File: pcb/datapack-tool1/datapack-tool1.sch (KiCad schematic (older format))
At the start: 4 parts

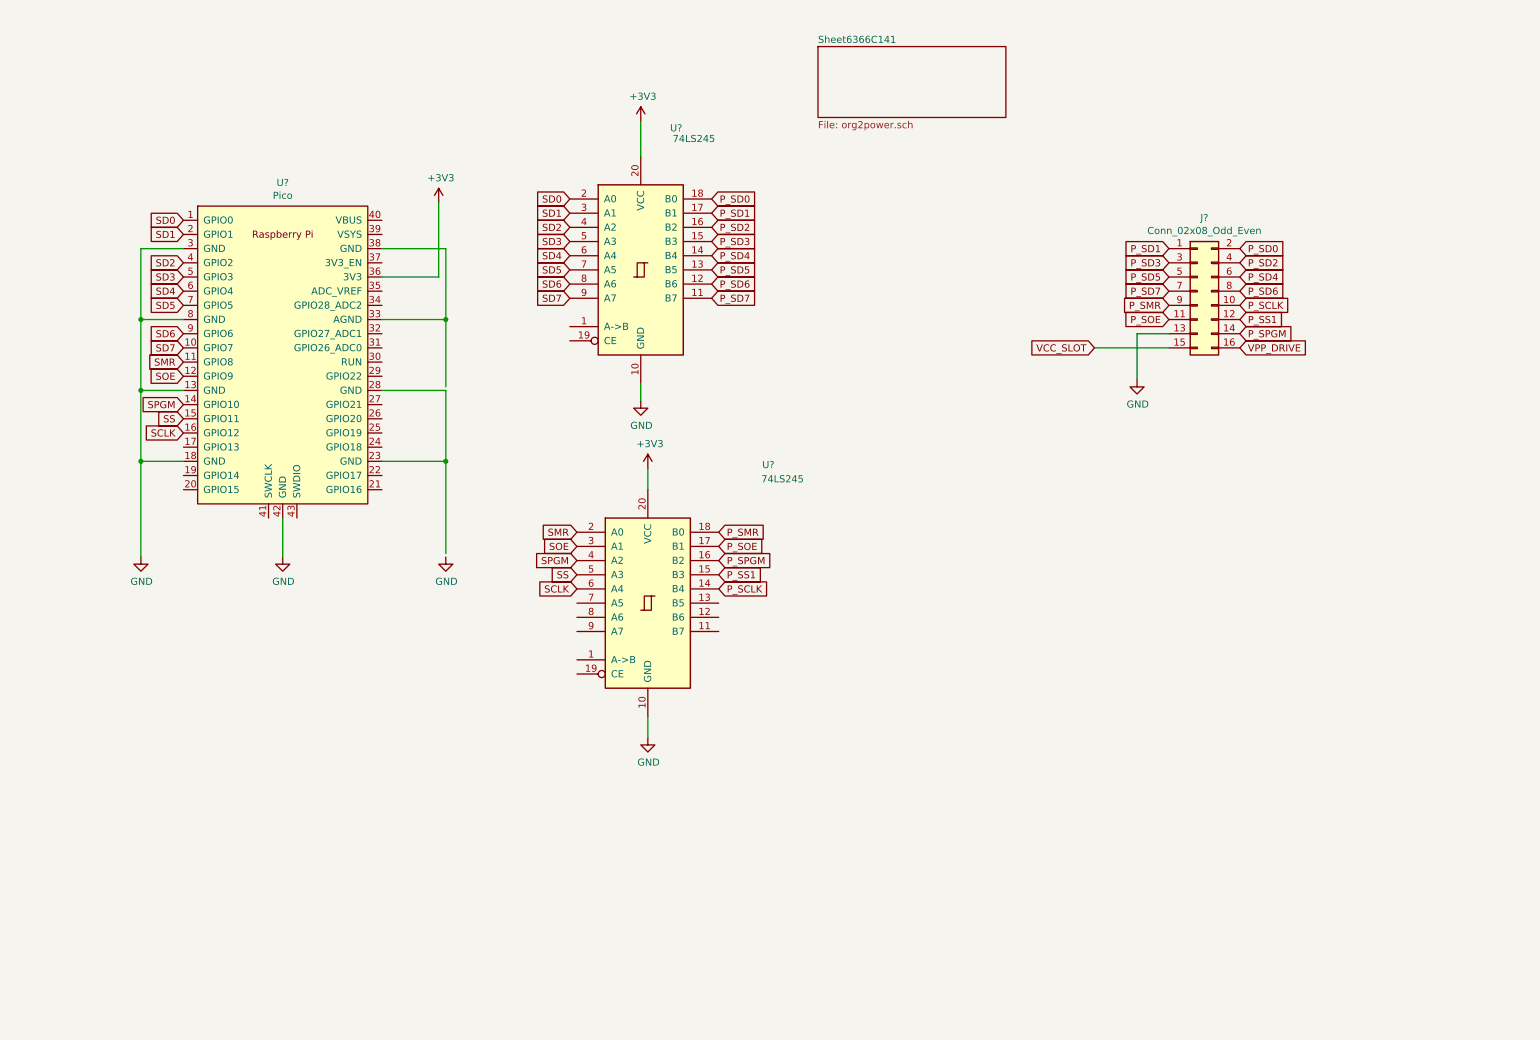
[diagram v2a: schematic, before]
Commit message: Updates
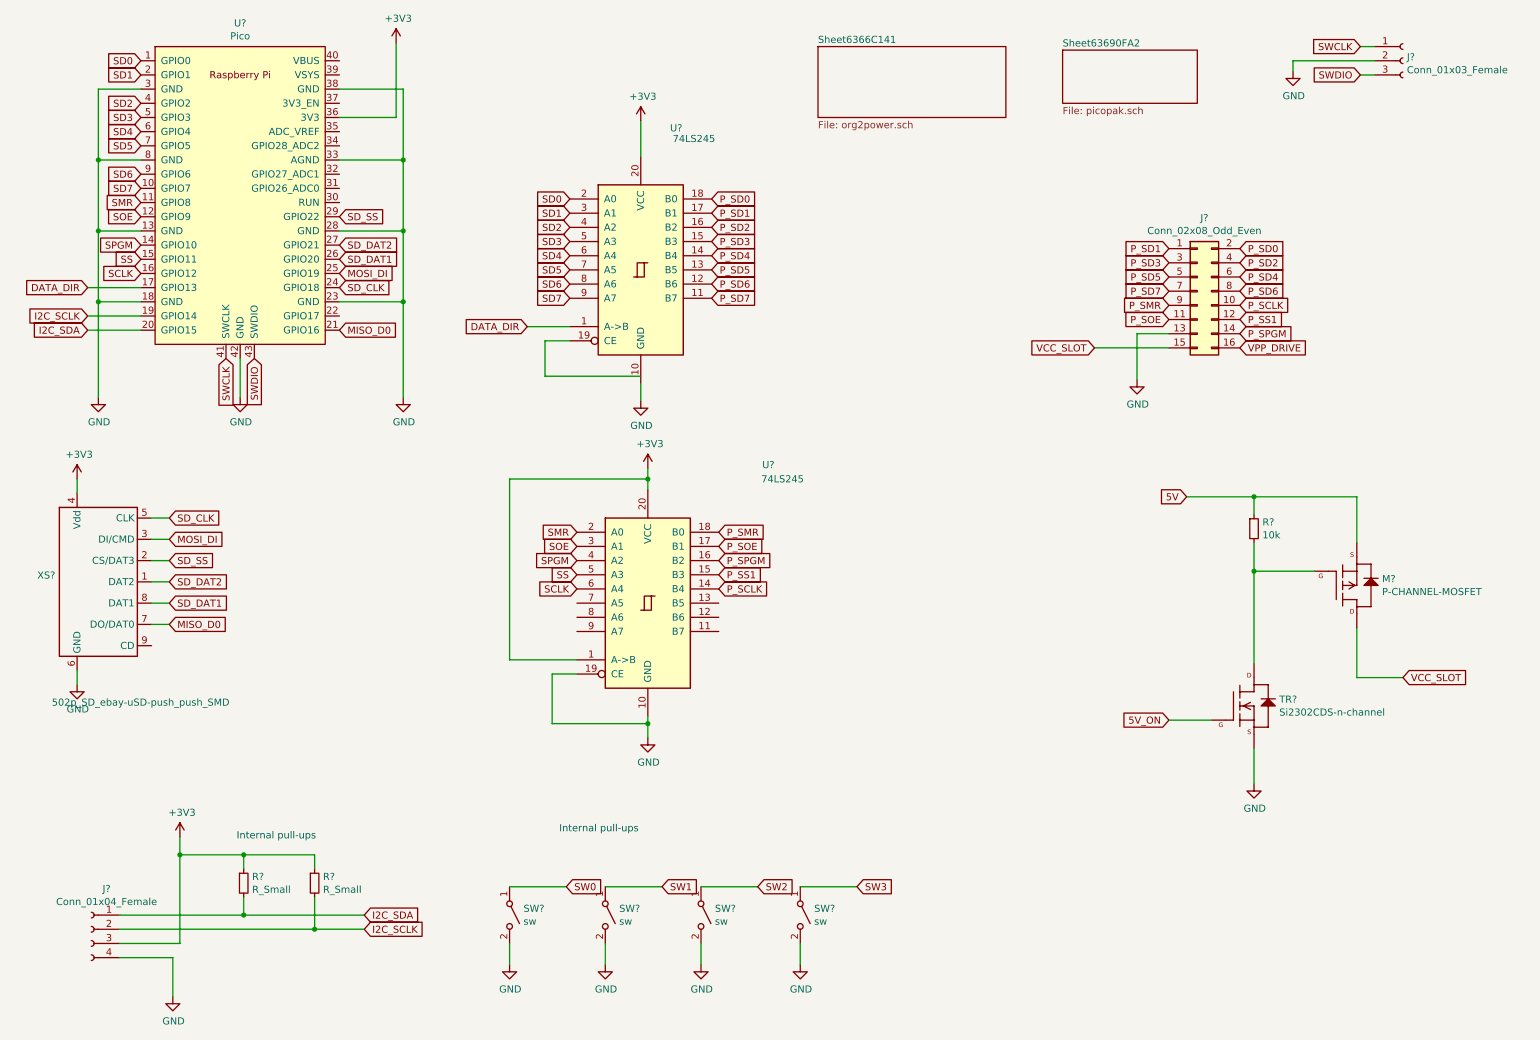
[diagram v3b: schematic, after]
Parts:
- added J?: Conn_01x04_Female, ajm_kicad:OLED_SMALL, symbol Connector:Conn_01x04_Female
- added J?: Conn_01x03_Female, symbol Connector:Conn_01x03_Female
- added M?: P-CHANNEL-MOSFET, Package_TO_SOT_SMD:SOT-23, symbol GeekAmmo:P-CHANNEL-MOSFET
- added R?: 10k, Resistor_SMD:R_0805_2012Metric, symbol Device:R_Small
- added R? (x2): R_Small, Capacitor_SMD:C_0402_1005Metric, symbol Device:R_Small
- added SW? (x4): sw, Button_Switch_SMD:SW_Push_1P1T_NO_Vertical_Wuerth_434133025816, symbol mirotan-due-cassette-shield-cache:Switch_SW_SPST
- added TR?: Si2302CDS-n-channel, Package_TO_SOT_SMD:SOT-23, symbol New_Library:Si2302CDS-n-channel
- added XS?: 502p_SD_ebay-uSD-push_push_SMD, Connectors:Conn_uSDcard, symbol pak_breakout:502p_SD_ebay-uSD-push_push_SMD
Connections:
- net labels added: 5V, 5V_ON, DATA_DIR, I2C_SCLK, I2C_SDA, MISO_D0, MOSI_DI, SD_CLK, SD_DAT1, SD_DAT2, SD_SS, SW0, SW1, SW2, SW3, SWCLK, SWDIO
- wire segments 26 -> 87
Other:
- note added: "Internal pull-ups"
- moved on the sheet: U?
